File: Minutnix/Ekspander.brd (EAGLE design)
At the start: 110.5 x 28.9 mm, 9 parts

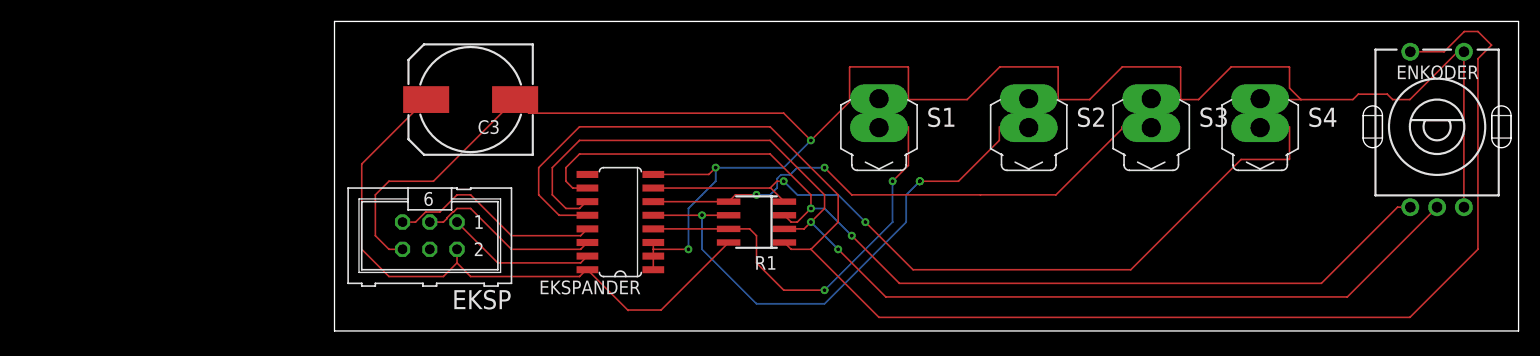
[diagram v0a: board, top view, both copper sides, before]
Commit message: Archivisation and actualisation
Archivisation of 1 version of boards
New version of boards
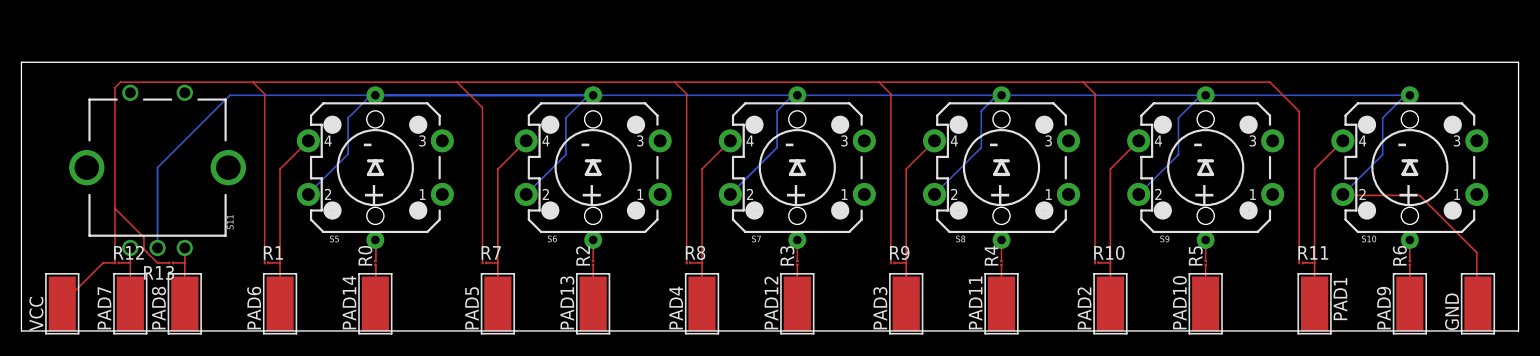
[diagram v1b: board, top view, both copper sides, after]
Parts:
- removed C3: (no value), rcl:140CLH-1010
- removed EKSP: (no value), con-harting-ml:ML6
- removed EKSPANDER: PCF8574AT, i2c:SO16
- removed ENKODER: CI-11, piher:CI-11
- removed S1, S2, S3, S4: (no value), switch:MS243
- added GND, PAD1, PAD10, PAD11, PAD12, PAD13, PAD14, PAD2, PAD3, PAD4, PAD5, PAD6, PAD7, PAD8, PAD9, VCC: WIREPADSMD5-2,5, wirepad:5-2,5
- added R0, R2, R3, R4, R5, R6: 220, rcl:R01005
- added R10, R11, R12, R13, R7, R8, R9: 4.7k, rcl:R01005
- added S10, S5, S6, S7, S8, S9: MOMENTARY-SWITCH-SPST-LED-PTH-12MM, SparkFun-Switches:TACTILE_SWITCH_LED_PTH_12MM
- added S11: ENCODER-SWITCH, SparkFun-Switches:ROTARY_ENC_PLAIN
- R1: value (none) -> 4.7k; device resistor-bourns:SO8 -> rcl:R01005
- moved R1 45.9 mm to (-3.81, 36.8), turned to 0 degrees
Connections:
- removed net GND: C3.-, EKSP.6, EKSPANDER.1, EKSPANDER.2, EKSPANDER.3, EKSPANDER.8, ENKODER.C, ENKODER.E, S1.2, S2.2, S3.2, S4.2
- new net N$12: PAD14.1, R0.1
- new net N$13: PAD1.1, R11.2, S10.4
- new net N$14: PAD8.1, R13.1, S11.B
- new net N$15: PAD7.1, R12.2, S11.A
- new net N$16: PAD6.1, R1.2, S5.4
- new net N$17: PAD5.1, R7.2, S6.4
- new net N$18: PAD4.1, R8.2, S7.4
- new net N$19: PAD3.1, R9.2, S8.4
- new net N$20: PAD2.1, R10.2, S9.4
- new net N$21: R1.1, R10.1, R11.1, R12.1, R13.2, R7.1, R8.1, R9.1, VCC.1
- new net N$85: GND.1, S10.2, S10.C, S11.C, S5.2, S5.C, S6.2, S6.C, S7.2, S7.C, S8.2, S8.C, S9.2, S9.C
- net N$1: now also R0.2, S5.A; no longer EKSP.5, EKSPANDER.13
- net N$10: now also PAD12.1, R3.1; no longer EKSPANDER.5, R1.6, S2.1
- net N$11: now also PAD13.1, R2.1; no longer EKSPANDER.4, R1.7, S1.1
- net N$2: now also R2.2, S6.A; no longer EKSP.1, EKSPANDER.15
- net N$3: now also R3.2, S7.A; no longer EKSP.3, EKSPANDER.14
- net N$4: now also R4.2, S8.A; no longer C3.+, EKSP.2, EKSPANDER.16, R1.8
- net N$5: now also R5.2, S9.A; no longer EKSPANDER.12, ENKODER.D, R1.1
- net N$6: now also R6.2, S10.A; no longer EKSPANDER.11, ENKODER.B, R1.2
- net N$7: now also PAD9.1, R6.1; no longer EKSPANDER.10, ENKODER.A, R1.3
- net N$8: now also PAD10.1, R5.1; no longer EKSPANDER.7, R1.4, S4.1
- net N$9: now also PAD11.1, R4.1; no longer EKSPANDER.6, R1.5, S3.1
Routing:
- net N$85: track 0.00 -> 280.8 mm
- net N$21: track 0.00 -> 243.8 mm
- net GND: track 182.0 -> 0.00 mm, vias 3 -> 0
- net N$5: track 144.9 -> 1.98 mm
- net N$6: track 105.8 -> 1.98 mm, vias 2 -> 0
- net N$7: track 94.8 -> 3.65 mm, vias 2 -> 0
- net N$8: track 72.2 -> 3.65 mm, vias 2 -> 0
- net N$4: track 58.6 -> 1.98 mm
- net N$9: track 49.3 -> 3.65 mm, vias 2 -> 0
- net N$10: track 49.1 -> 3.65 mm, vias 3 -> 0
- net N$11: track 38.3 -> 3.65 mm, vias 2 -> 0
- net N$1: track 20.1 -> 2.01 mm
- net N$19: track 0.00 -> 17.4 mm
- net N$18: track 0.00 -> 17.4 mm
- net N$17: track 0.00 -> 17.4 mm
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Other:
- board size 110.5 x 28.9 mm -> 139.7 x 25.1 mm
